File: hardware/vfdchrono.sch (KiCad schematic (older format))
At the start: 2 parts, among them U3 IVL2-5_7, U4 HV5812WG

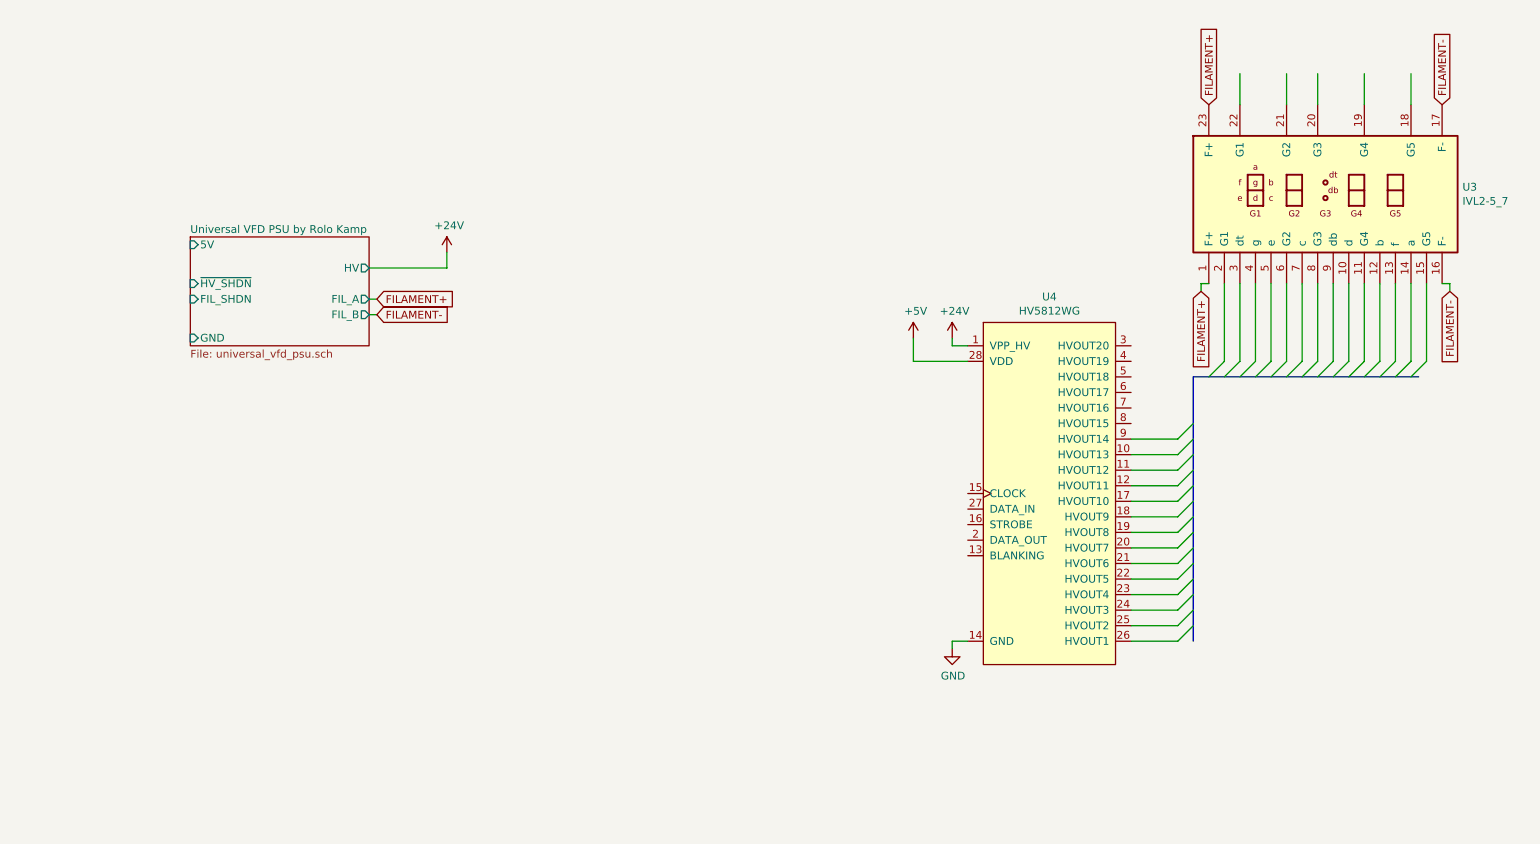
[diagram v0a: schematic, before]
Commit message: commit the board version that went to aisler, more silkscreen info
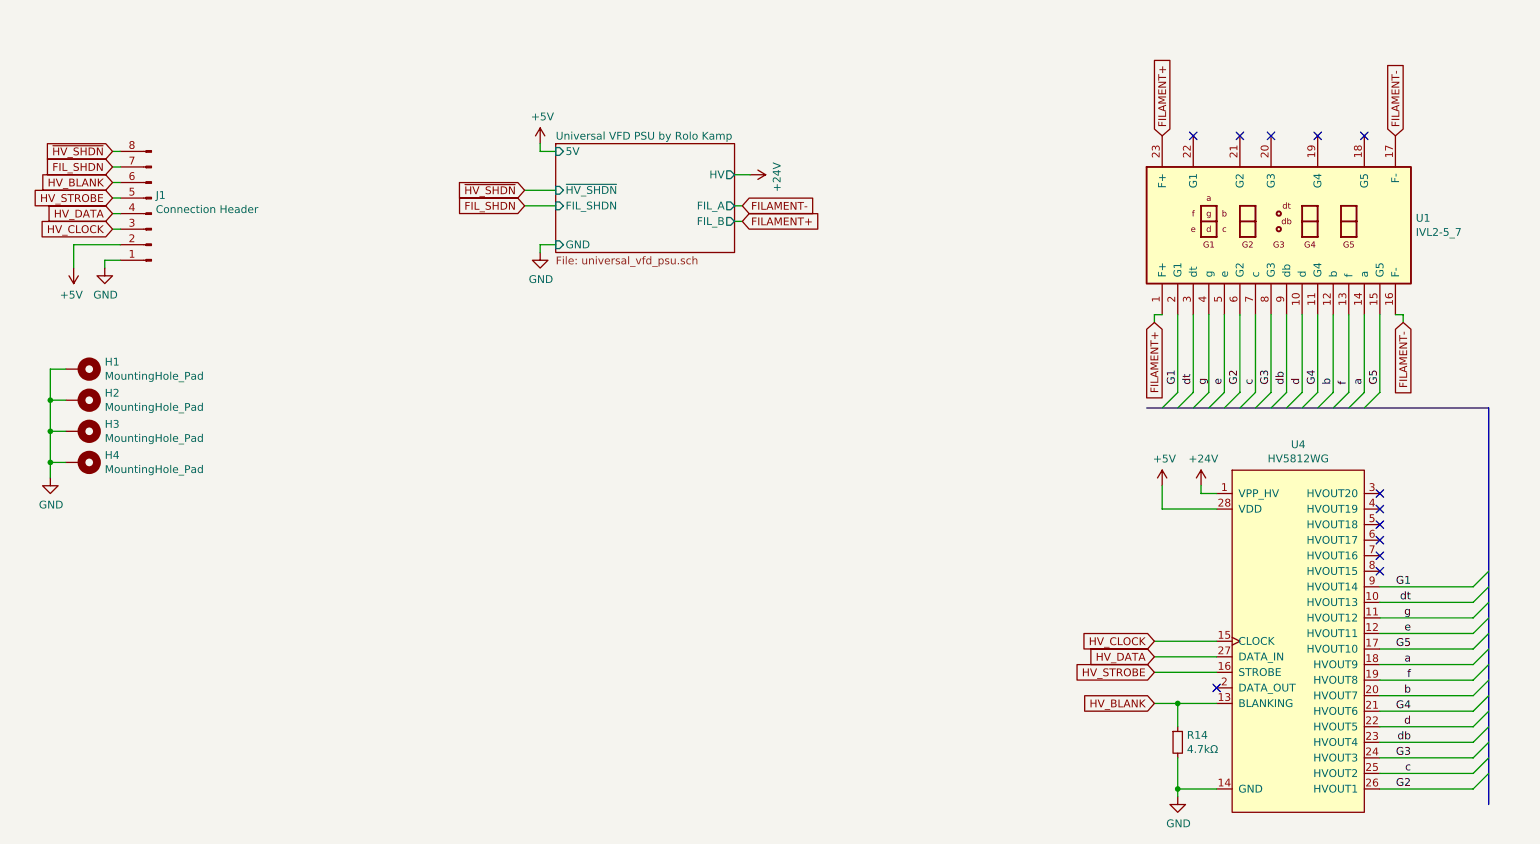
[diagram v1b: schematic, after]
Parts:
- added H1, H2, H3, H4: MountingHole_Pad, MountingHole:MountingHole_2.7mm_M2.5_Pad, symbol Mechanical:MountingHole_Pad
- added J1: Connection Header, Connector_PinHeader_2.54mm:PinHeader_1x08_P2.54mm_Vertical, symbol Connector:Conn_01x08_Male
- added R14: 4.7kΩ, Resistor_SMD:R_0805_2012Metric_Pad1.15x1.40mm_HandSolder, symbol Device:R_Small
- renumbered U3 to U1
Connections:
- net labels added: FIL_SHDN, G1, G2, G3, G4, G5, HV_BLANK, HV_CLOCK, HV_DATA, HV_STROBE, a, b, c, d, db, dt, e, f, g, ~HV_SHDN~
- wire segments 47 -> 72
- no-connect marks 0 -> 12
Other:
- moved on the sheet: U1, U4
